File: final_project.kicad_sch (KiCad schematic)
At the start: 5 parts, among them U1 ATmega328-P, U2 SGP30

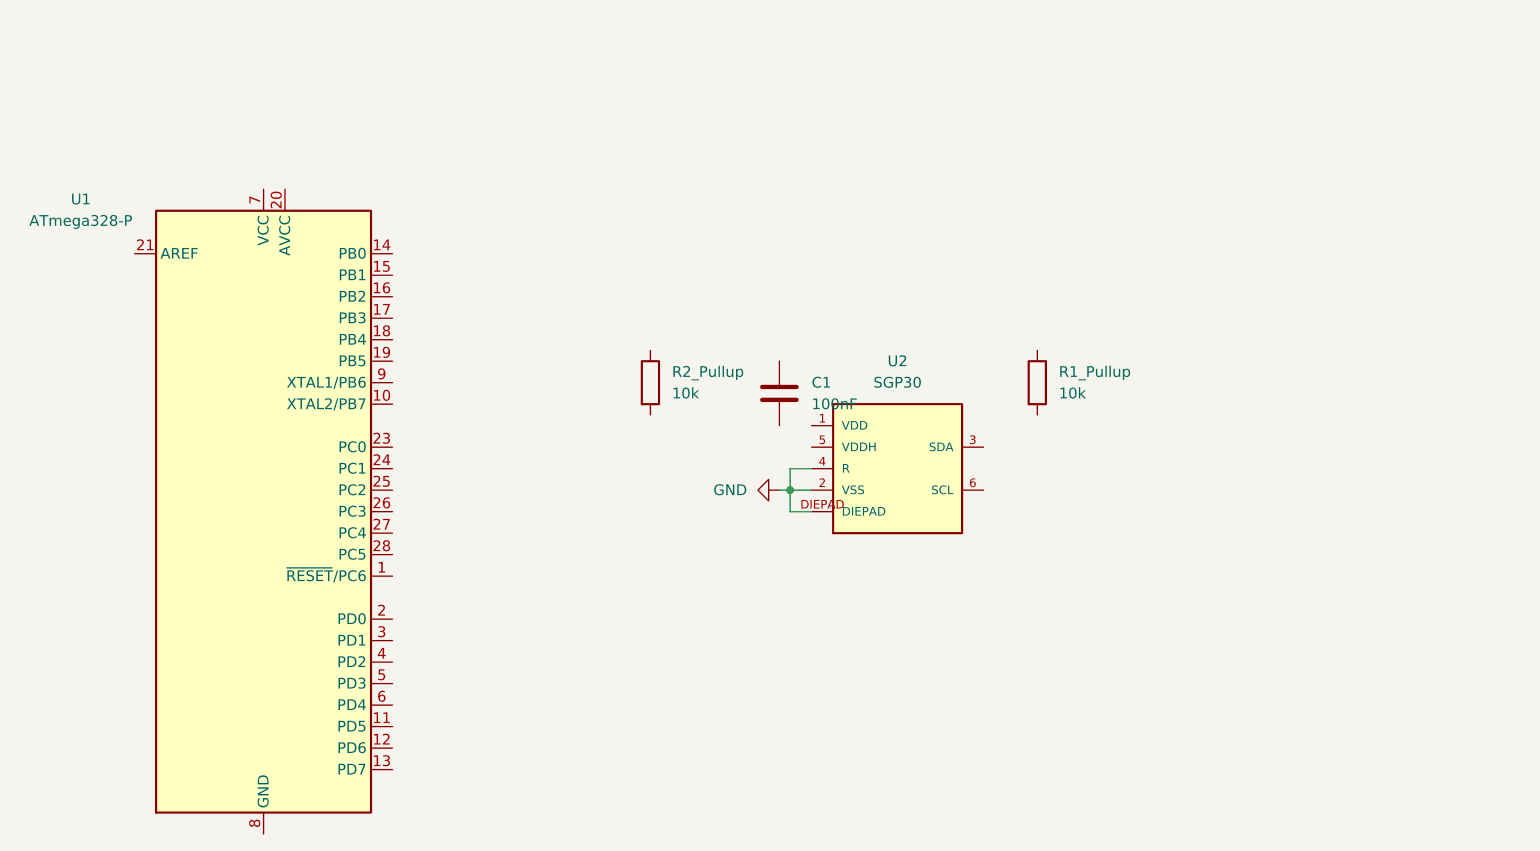
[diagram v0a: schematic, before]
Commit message: Added Voltage Regulator
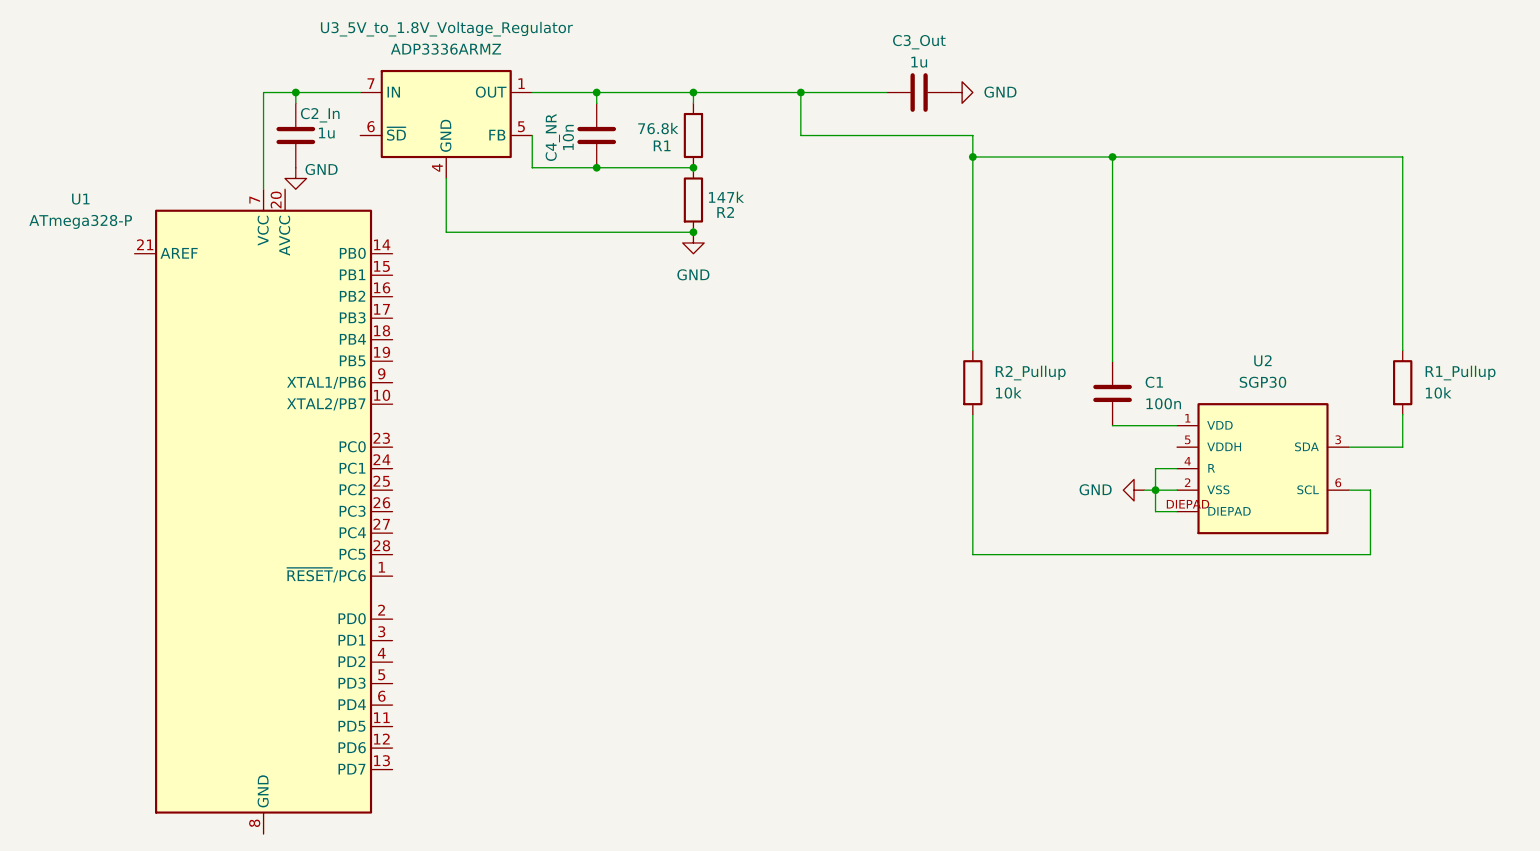
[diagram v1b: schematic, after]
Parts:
- added C2_In, C3_Out: 1u, symbol Device:C
- added C4_NR: 10n, symbol Device:C
- added R1: 76.8k, symbol Device:R
- added R2: 147k, symbol Device:R
- added U3_5V_to_1.8V_Voltage_Regulator: ADP3336ARMZ, Package_SO:MSOP-8_3x3mm_P0.65mm, symbol Regulator_Linear:ADP3336ARMZ
- C1: value 100nF -> 100n
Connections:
- net GND: now also C2_In.2, C3_Out.2, R2.2, U3_5V_to_1.8V_Voltage_Regulator.4 (GND)
- net at C1.1: now also R1_Pullup.1, R2_Pullup.1, C3_Out.1, C4_NR.2, R1.2, U3_5V_to_1.8V_Voltage_Regulator.1 (OUT), U3_5V_to_1.8V_Voltage_Regulator.2 (OUT), U3_5V_to_1.8V_Voltage_Regulator.3 (OUT)
- net at C1.2: now also U2.1 (VDD)
- net at U2.3 (SDA): now also R1_Pullup.2
- net at U2.6 (SCL): now also R2_Pullup.2
- net at U1.7 (VCC): now also C2_In.1, U3_5V_to_1.8V_Voltage_Regulator.7 (IN), U3_5V_to_1.8V_Voltage_Regulator.8 (IN)
- new net: C4_NR.1, R1.1, R2.1, U3_5V_to_1.8V_Voltage_Regulator.5 (FB)
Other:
- moved on the sheet: C1, R1_Pullup, R2_Pullup, U2
